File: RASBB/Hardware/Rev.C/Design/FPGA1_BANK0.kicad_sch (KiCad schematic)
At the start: 16 parts, among them J13 Conn_01x06_Socket, U10 XC7A100T-CSG324

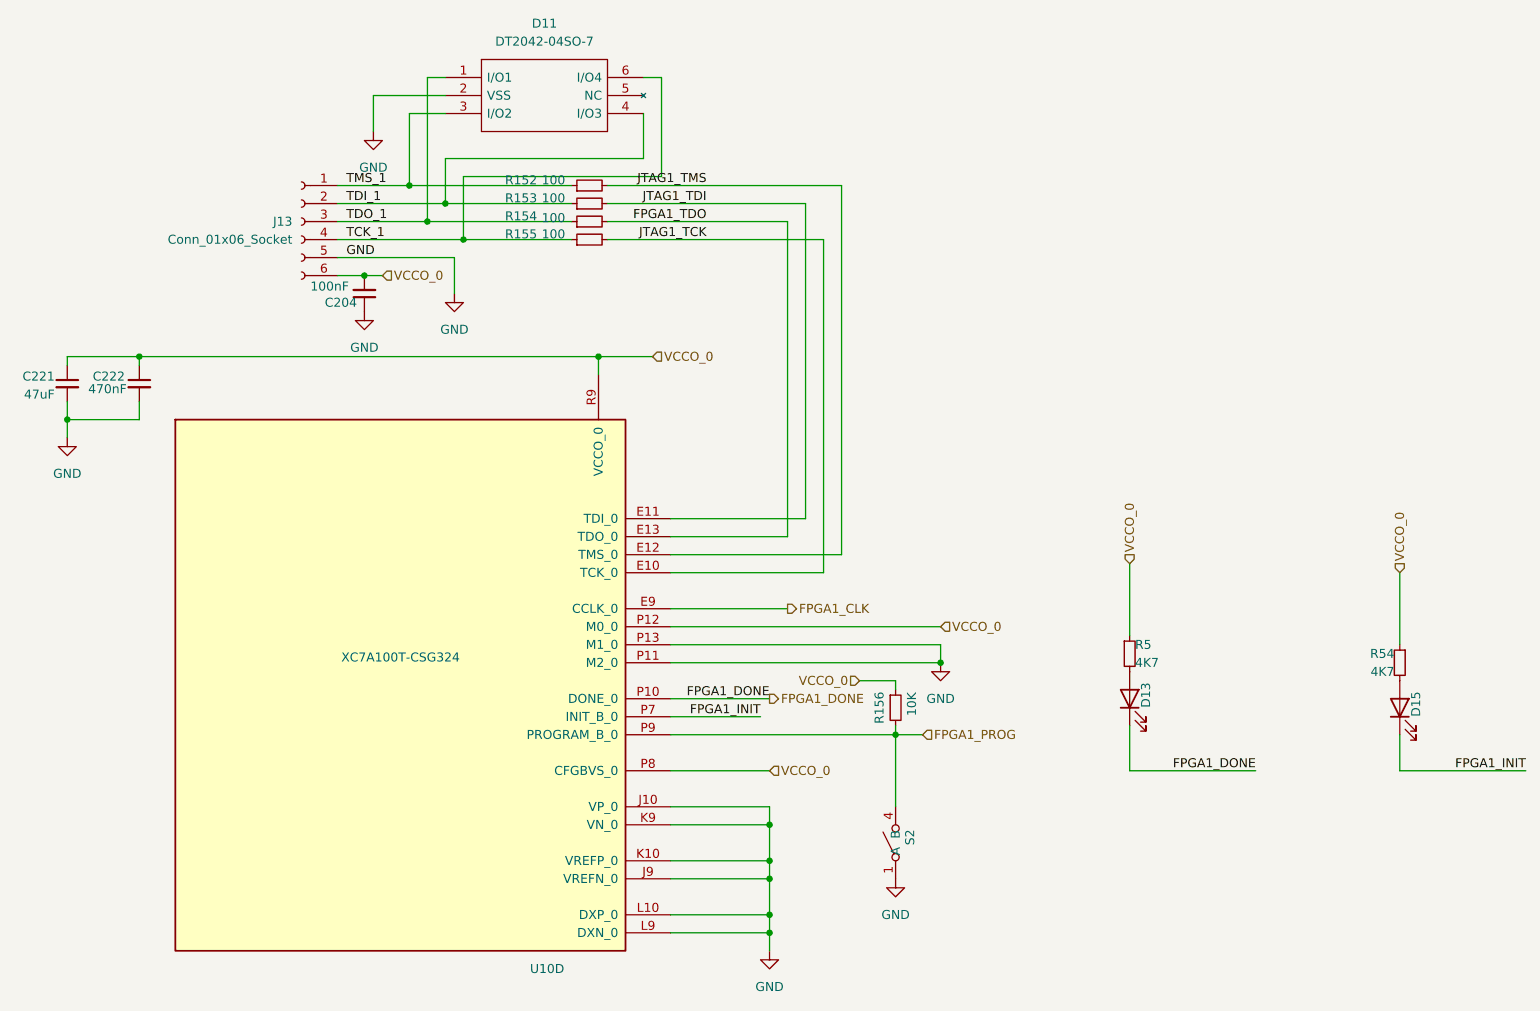
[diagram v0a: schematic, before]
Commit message: Draft AC
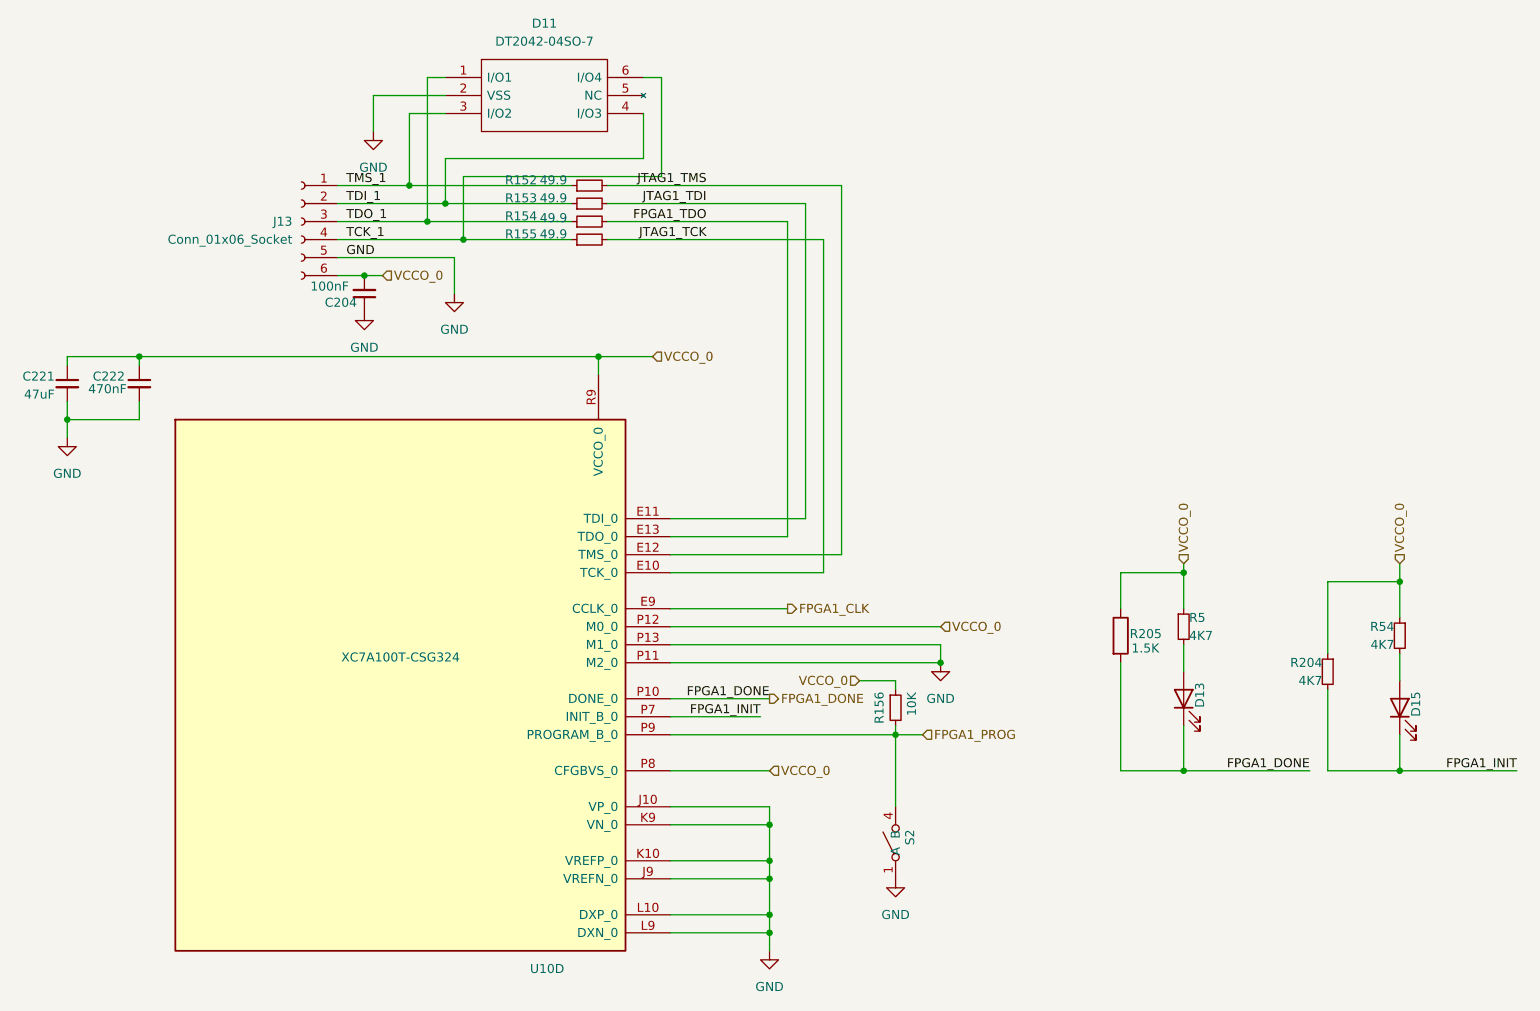
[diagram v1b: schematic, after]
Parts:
- added R204: 4K7, Resistor_SMD:R_0402_1005Metric, symbol Device:R_Small
- added R205: 1.5K, Resistor_SMD:R_0402_1005Metric, symbol Device:R
- R152, R153, R154, R155: value 100 -> 49.9; LCSC Part # C163808 -> C4229190; Mfr. Part # WR04X1000FTL -> RMCF0402FT49R9
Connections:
- net FPGA1_DONE: now also R205.2
- net FPGA1_INIT: now also R204.2
- net VCCO_0: now also R204.1, R205.1
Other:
- moved on the sheet: D13, R5, R54

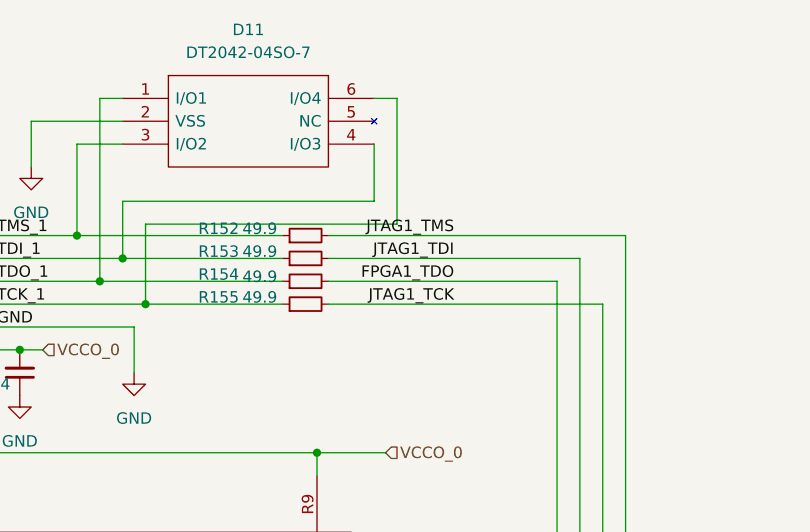
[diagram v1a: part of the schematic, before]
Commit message: Modified Based on Findings -Draft
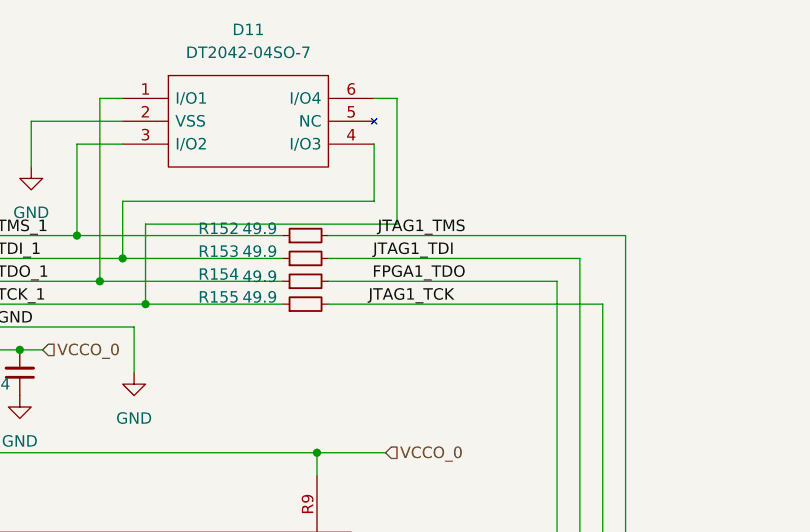
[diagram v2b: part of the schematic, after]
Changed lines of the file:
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@@
 	(title_block
 		(title "RASBB")
-		(date "2026-07-25")
+		(date "2026-09-20")
 		(rev "C")
 		(company "Mina Daneshpajouh")
@@
 	)
 	(label "JTAG1_TMS"
-		(at 130.81 41.91 180)
+		(at 132.08 41.91 180)
 		(effects
 			(font
@@
 	)
 	(label "FPGA1_TDO"
-		(at 130.81 46.99 180)
+		(at 132.08 46.99 180)
 		(effects
 			(font
